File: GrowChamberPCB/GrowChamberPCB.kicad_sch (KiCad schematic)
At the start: 5 parts, among them CN2 RelayBoard Interconnect, P1 To Faceplate, U4 To Faceplate, U6 CR2013-MI2120

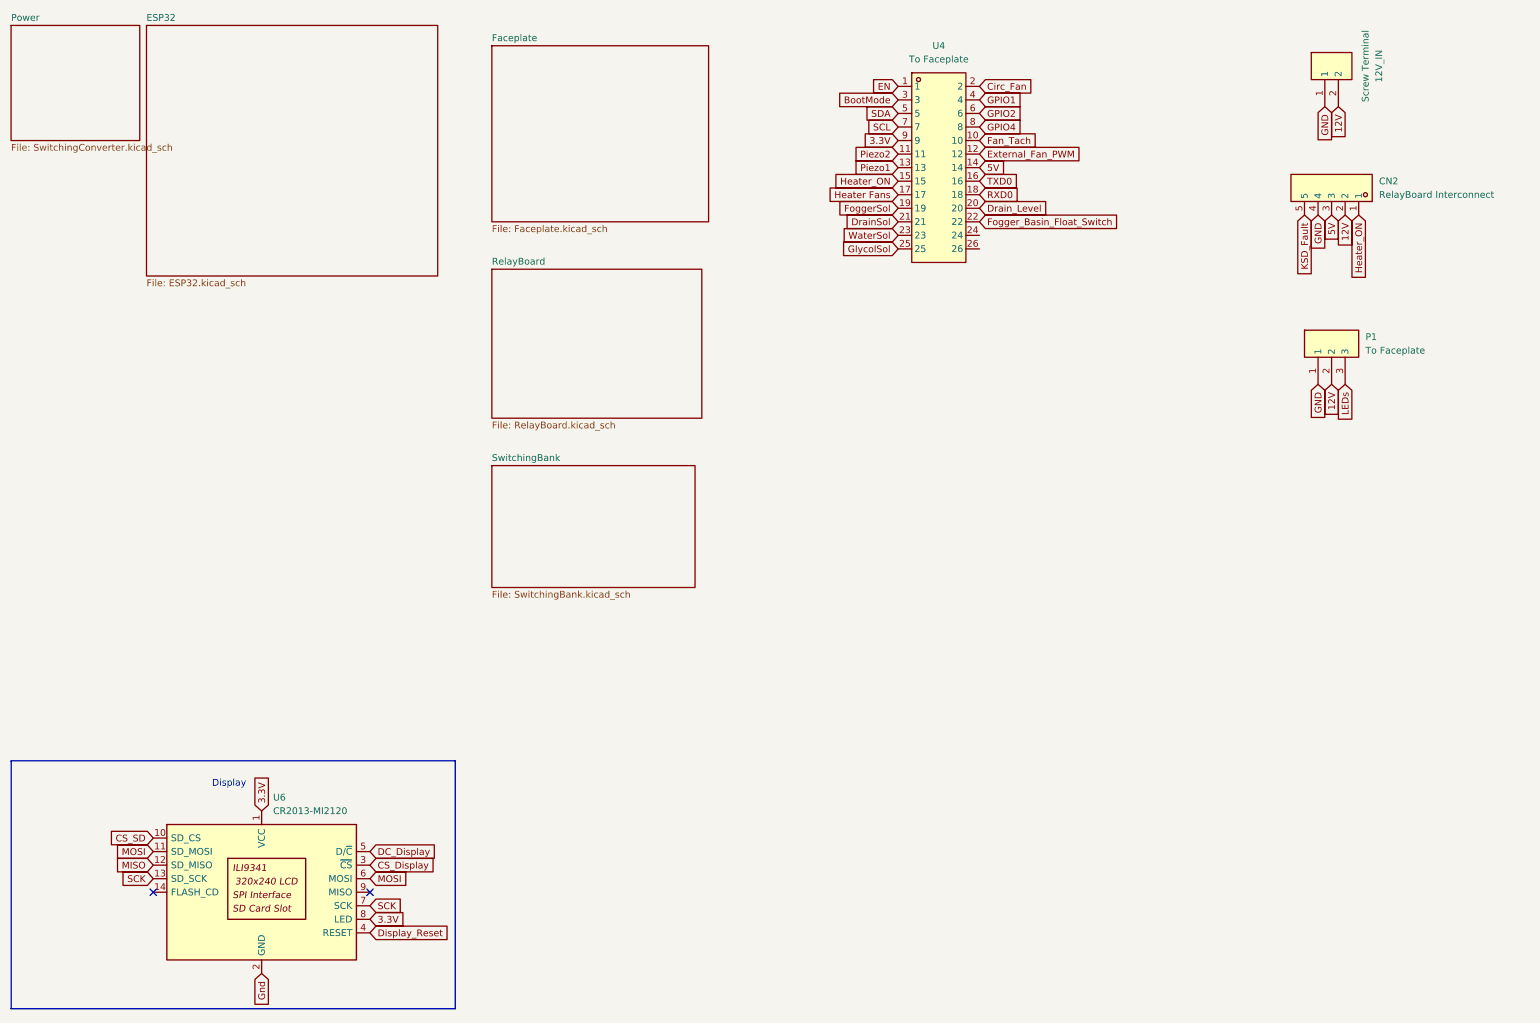
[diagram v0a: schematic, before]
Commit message: almost done!
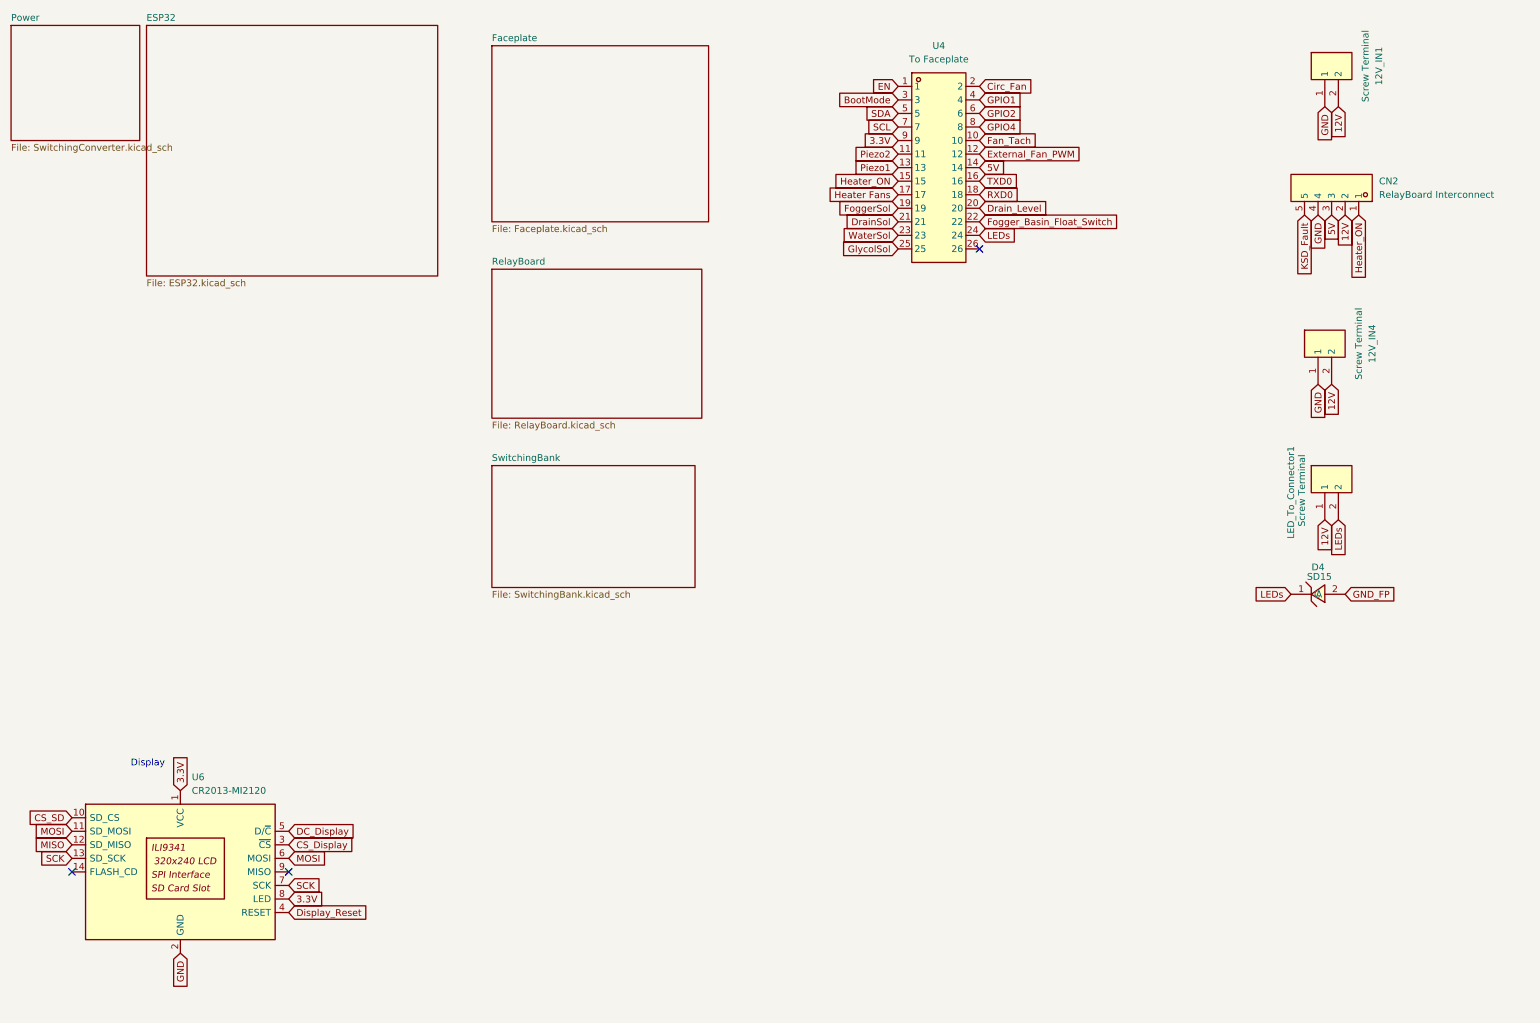
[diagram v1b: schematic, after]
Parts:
- removed P1: To Faceplate, easyeda2kicad:CONN-TH_3P-P5.00_WJ127-5.0-3P, symbol easyeda2kicad:WJ127-5.0-3P
- added 12V_IN4, LED_To_Connector1: Screw Terminal, easyeda2kicad:CONN-TH_2P-P5.00_CPC3703CTR, symbol easyeda2kicad:WJ127-5.0-2P
- added D4: SD15, easyeda2kicad:SOD-323_L1.7-W1.3-LS2.6-RD, symbol easyeda2kicad:SD15_C2931147
- renumbered 12V_IN to 12V_IN1
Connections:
- net Gnd is gone; now on net GND: U6.2 (GND)
- net 12V: now also 12V_IN4.2, LED_To_Connector1.1
- net GND: now also 12V_IN4.1
- net LEDs: now also U4.24, D4.1 (C), LED_To_Connector1.2
- new net GND_FP: D4.2 (A)
- no-connect marks 2 -> 3
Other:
- moved on the sheet: U6
